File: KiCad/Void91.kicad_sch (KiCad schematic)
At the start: 1 part

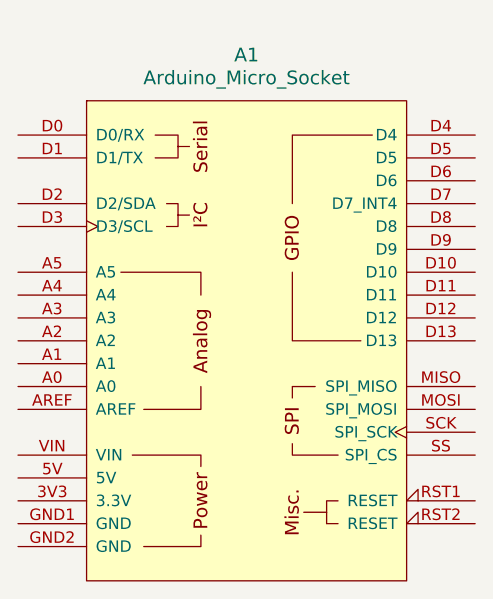
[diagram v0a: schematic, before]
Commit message: .
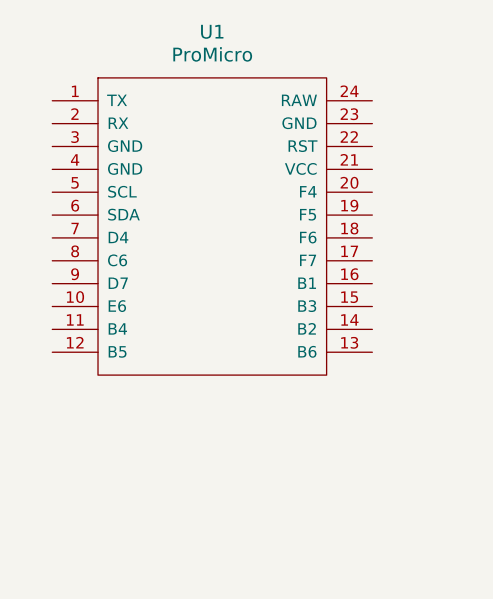
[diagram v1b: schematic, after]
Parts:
- removed A1: Arduino_Micro_Socket, PCM_arduino-library:Arduino_Micro_Socket, symbol PCM_arduino-library:Arduino_Micro_Socket
- added U1: ProMicro, Keebio-Parts:ArduinoProMicro, symbol promicro:ProMicro
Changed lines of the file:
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@@
 (kicad_sch (version 20230121) (generator eeschema)
   (paper "A4")
-  (symbol (lib_id "PCM_arduino-library:Arduino_Micro_Socket") (at 68.58 83.82 0) (unit 1)
+  (symbol (lib_id "promicro:ProMicro") (at 64.77 76.2 0) (unit 1)
     (in_bom yes) (on_board yes) (dnp no) (fields_autoplaced)
-    (property "Reference" "A1" (at 68.58 52.07 0)
+    (property "Reference" "U1" (at 64.77 49.53 0)
       (effects (font (size 1.524 1.524)))
     )
-    (property "Value" "Arduino_Micro_Socket" (at 68.58 54.61 0)
+    (property "Value" "ProMicro" (at 64.77 52.07 0)
       (effects (font (size 1.524 1.524)))
     )
-    (property "Footprint" "PCM_arduino-library:Arduino_Micro_Socket" (at 68.58 118.11 0)
+    (property "Footprint" "Keebio-Parts:ArduinoProMicro" (at 67.31 102.87 0)
       (effects (font (size 1.524 1.524)) hide)
     )
-    (property "Datasheet" "https://docs.arduino.cc/hardware/micro" (at 68.58 114.3 0)
-      (effects (font (size 1.524 1.524)) hide)
+    (property "Datasheet" "" (at 67.31 102.87 0)
+      (effects (font (size 1.524 1.524)))
     )
-    (pin "D10")
-    (pin "A1")
-    (pin "D2")
-    (pin "D1")
-    (pin "D3")
-    (pin "3V3")
-    (pin "5V")
-    (pin "D5")
-    (pin "D9")
-    (pin "A3")
-    (pin "D0")
-    (pin "GND1")
-    (pin "MOSI")
-    (pin "A2")
-    (pin "A5")
-    (pin "D11")
-    (pin "D12")
-    (pin "D6")
-    (pin "D8")
-    (pin "GND2")
-    (pin "A4")
-    (pin "AREF")
-    (pin "MISO")
-    (pin "RST1")
-    (pin "A0")
-    (pin "D13")
-    (pin "D4")
-    (pin "D7")
-    (pin "RST2")
-    (pin "VIN")
-    (pin "SS")
-    (pin "SCK")
+    (pin "22")
+    (pin "23")
+    (pin "4")
+    (pin "9")
+    (pin "13")
+    (pin "2")
+    (pin "1")
+    (pin "14")
+    (pin "15")
+    (pin "20")
+    (pin "19")
+    (pin "6")
+    (pin "8")
+    (pin "3")
+    (pin "18")
+    (pin "11")
+    (pin "12")
+    (pin "7")
+    (pin "5")
+    (pin "24")
+    (pin "17")
+    (pin "21")
+    (pin "16")
+    (pin "10")
     (instances
       (project "Void91"
         (path "/7e6e1662-906b-4325-9d43-4b425f9d2cd5"
-          (reference "A1") (unit 1)
+          (reference "U1") (unit 1)
         )
       )
